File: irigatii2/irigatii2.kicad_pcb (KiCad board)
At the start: 2 copper layers, 100 x 100 mm, 108 parts, among them IC1 MIC3172YN, IC2 PCA9575PW2,118, J2 Conn_01x05, J5 valve, J6 valve, J7 valve, J8 valve, J9 valve, Q11 PMOS, Q12 PMOS, Q13 PMOS, Q14 PMOS, Q15 NMOS, Q16 NMOS, Q17 NMOS, Q18 NMOS, Q19 NMOS, Q20 NMOS, Q21 NMOS, Q22 NMOS, Q23 PMOS, Q24 PMOS, Q25 PMOS, Q26 PMOS, Q27 NMOS, Q28 NMOS, Q29 NMOS, Q30 NMOS, Q31 NMOS, Q32 NMOS, Q33 NMOS, Q34 NMOS, Q35 PMOS, Q36 PMOS, Q37 NMOS, Q38 NMOS, T1 Transformer_1P_1S, U1 NJM2114, U2 TL431LP

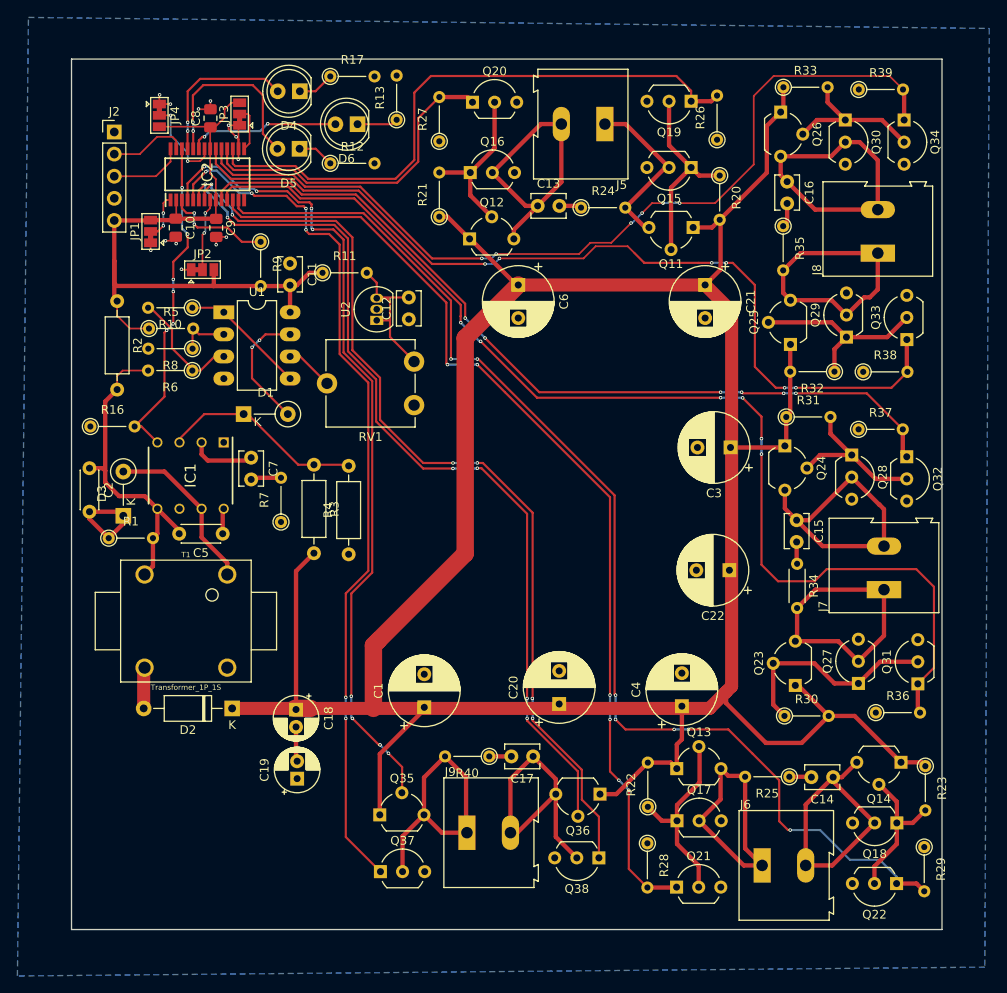
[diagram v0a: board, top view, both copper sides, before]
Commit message: v
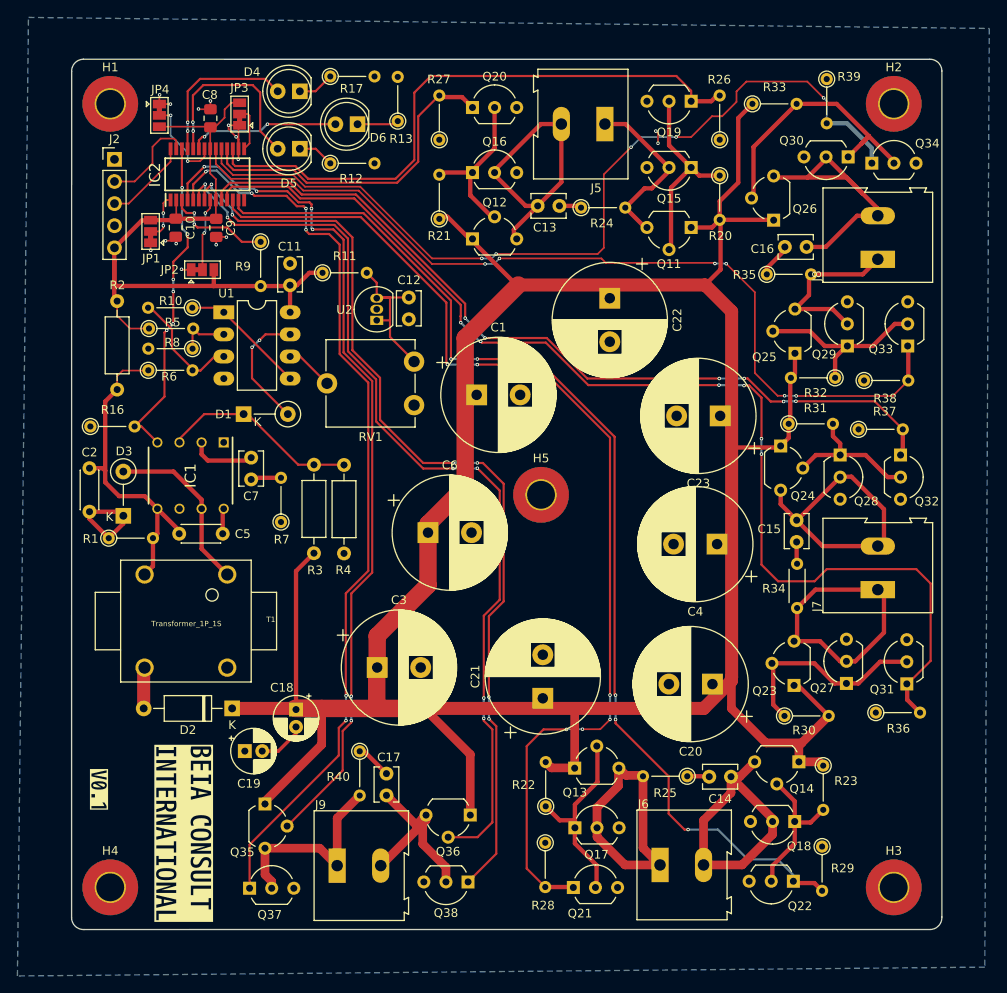
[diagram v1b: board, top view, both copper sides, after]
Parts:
- added C23: 500+u, Capacitor_THT:CP_Radial_D13.0mm_P5.00mm, F.Cu at (102.1, 121.8)
- added H1: MountingHole_Pad, MountingHole:MountingHole_3.2mm_M3_Pad_TopBottom, F.Cu at (32.0, 86.0)
- added H2: MountingHole_Pad, MountingHole:MountingHole_3.2mm_M3_Pad_TopBottom, F.Cu at (122.0, 86.0)
- added H3: MountingHole_Pad, MountingHole:MountingHole_3.2mm_M3_Pad_TopBottom, F.Cu at (122.0, 176.0)
- added H4: MountingHole_Pad, MountingHole:MountingHole_3.2mm_M3_Pad_TopBottom, F.Cu at (32.0, 176.0)
- added H5: MountingHole_Pad, MountingHole:MountingHole_3.2mm_M3_Pad_TopBottom, F.Cu at (81.5, 130.9)
- added kibuzzard-633BE47A: G***, kibuzzard-633BE47A, F.Cu at (40.4, 169.8)
- added kibuzzard-633BE88B: G***, kibuzzard-633BE88B, F.Cu at (30.7, 164.7)
- C1, C20, C21, C22, C3, C4, C6: value 220u -> 500+u; footprint Capacitor_THT:CP_Radial_D8.0mm_P3.80mm -> Capacitor_THT:CP_Radial_D13.0mm_P5.00mm
- moved C21 51.0 mm to (81.7, 154.3), turned to 90 degrees
- moved C3 47.8 mm to (62.7, 150.7), turned to 0 degrees
- moved C1 36.4 mm to (74.1, 119.4), turned to 0 degrees
- moved C22 34.1 mm to (89.4, 108.3), turned to -90 degrees
- moved C6 30.3 mm to (68.5, 135.3), turned to 0 degrees
- moved C4 19.1 mm to (101.7, 136.6), turned to 180 degrees
- moved C20 17.8 mm to (101.2, 152.7), turned to 180 degrees
- moved C17 17.4 mm to (63.7, 165.4), turned to 90 degrees
- moved J9 15.4 mm to (58.1, 173.5)
- moved Q38 15.3 mm to (73.1, 175.4)
- moved Q37 15.2 mm to (48.0, 176.1)
- moved Q36 15.1 mm to (73.4, 167.7)
- moved R40 14.9 mm to (60.7, 160.4), turned to -90 degrees
- moved Q35 13.2 mm to (49.8, 166.4), turned to -90 degrees
- moved Q26 12.4 mm to (108.2, 99.4), turned to 90 degrees
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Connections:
- R6 pad 1: Net-(R10-Pad2) -> Net-(C2-Pad1)
- R6 pad 2: Net-(C2-Pad1) -> Net-(R10-Pad2)
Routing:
- net Net-(Q26-Pad2): track 18.0 -> 31.7 mm
- net Net-(J8-Pad1): track 31.6 -> 19.9 mm
- net D1_1: track 112.1 -> 123.0 mm
- net D1_2: track 134.4 -> 126.6 mm, vias 7 -> 5
- net Net-(J9-Pad1): track 30.8 -> 23.2 mm
- net Net-(C17-Pad1): track 30.6 -> 23.3 mm
- net D3_2: track 100.4 -> 105.3 mm
- net D3_1: track 94.1 -> 98.5 mm, vias 8 -> 6
- net D3_3: track 103.1 -> 106.8 mm
- net I2C_SDA: track 9.06 -> 11.3 mm
- net D2_1: track 129.1 -> 131.0 mm
- net +3V3: track 83.4 -> 81.5 mm
- net Net-(Q24-Pad2): track 18.6 -> 16.8 mm
- net Net-(C17-Pad2): track 2.53 -> 4.13 mm
- net GND: track 22.3 -> 23.8 mm, vias 13 -> 15
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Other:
- outline, holes or cut-outs redrawn
